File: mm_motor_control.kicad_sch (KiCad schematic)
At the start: 0 parts

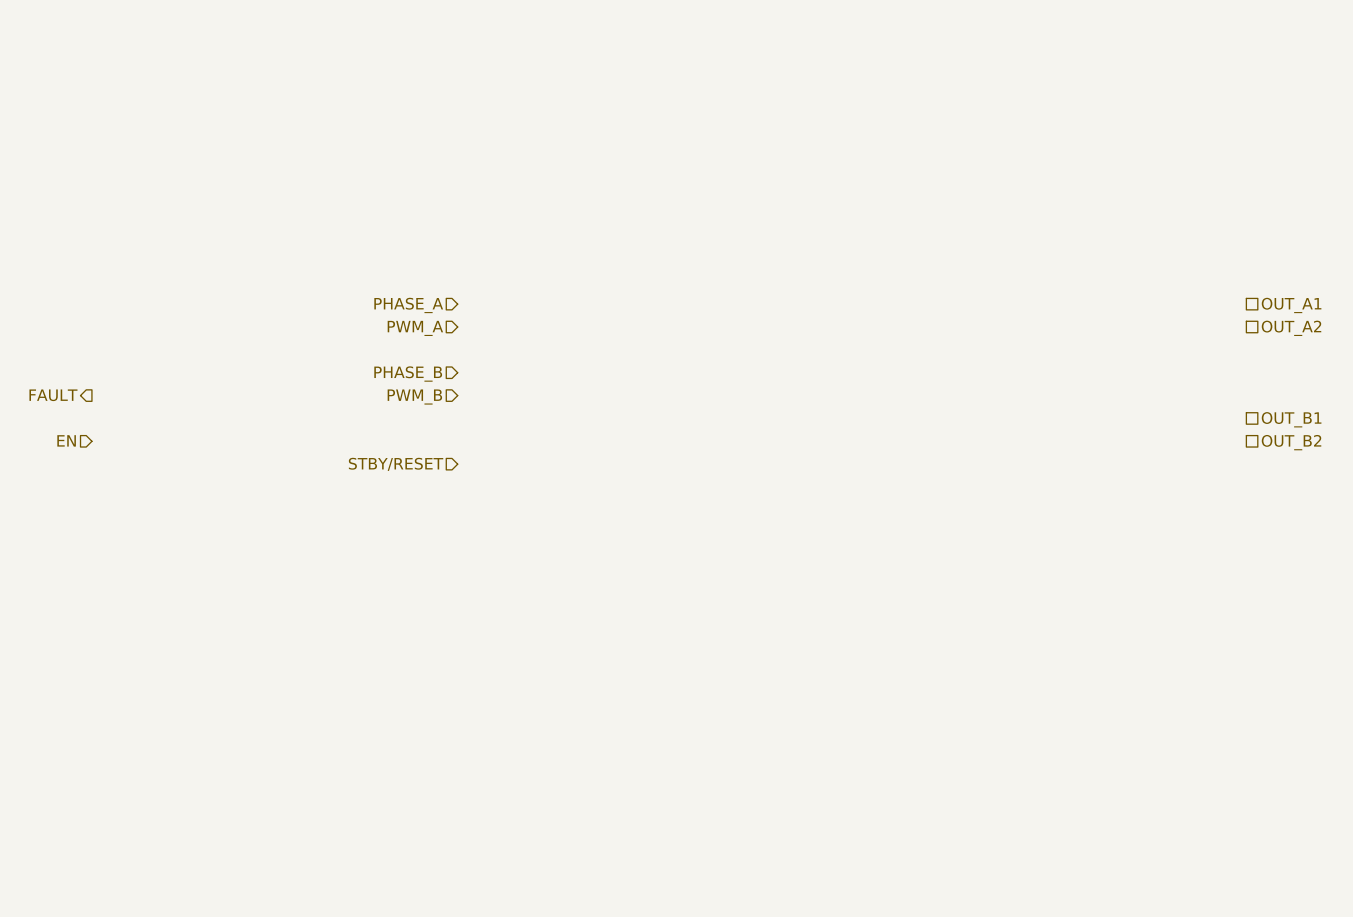
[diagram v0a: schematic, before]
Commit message: fin TP2
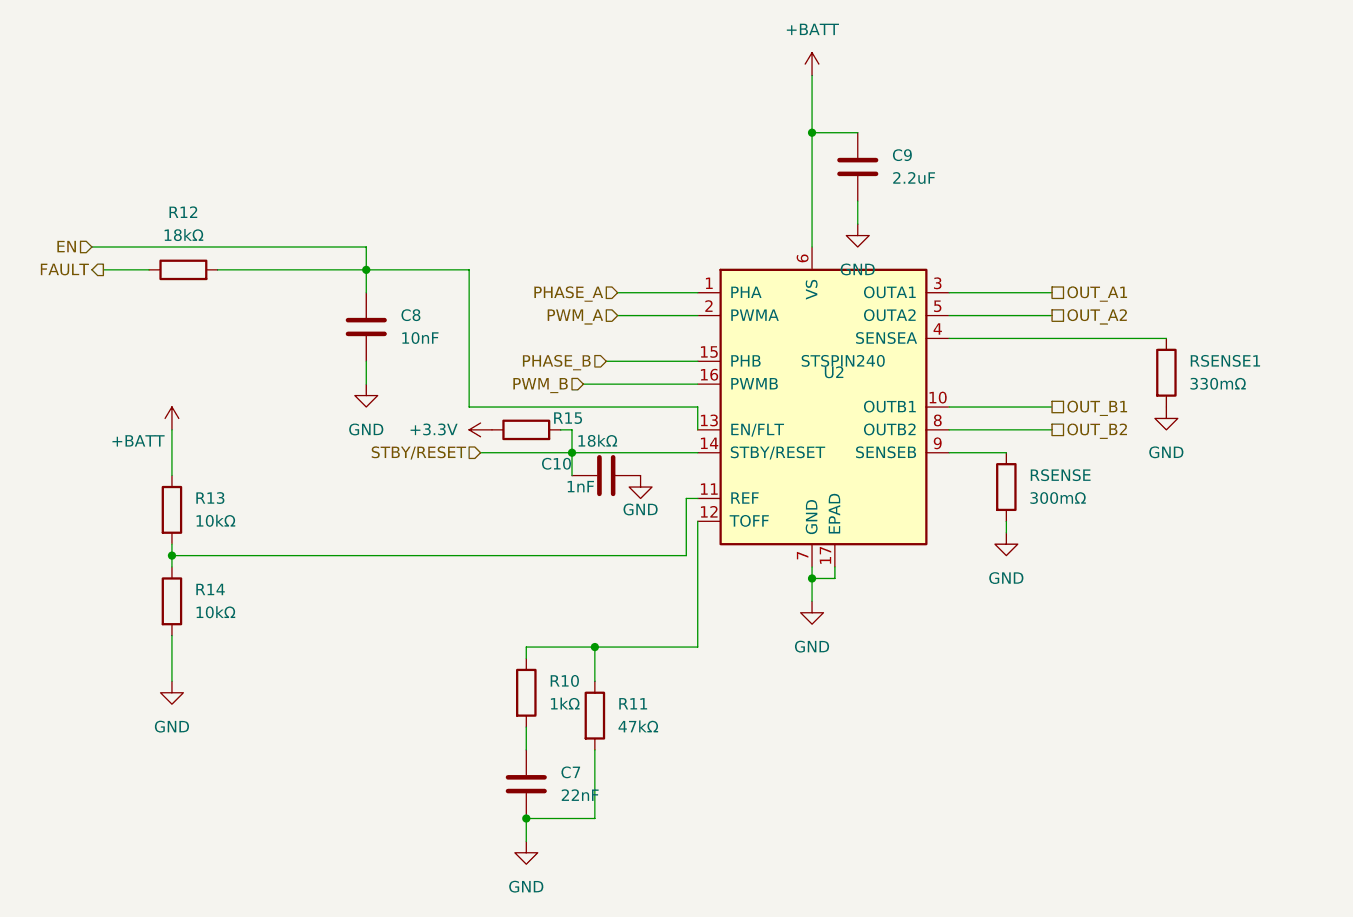
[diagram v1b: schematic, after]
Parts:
- added C10: 1nF, Capacitor_SMD:C_0603_1608Metric, symbol Device:C
- added C7: 22nF, Capacitor_SMD:C_0603_1608Metric, symbol Device:C
- added C8: 10nF, Capacitor_SMD:C_0603_1608Metric, symbol Device:C
- added C9: 2.2uF, Capacitor_SMD:C_0603_1608Metric, symbol Device:C
- added R10: 1kΩ, Resistor_SMD:R_0603_1608Metric, symbol Device:R
- added R11: 47kΩ, Resistor_SMD:R_0603_1608Metric, symbol Device:R
- added R12, R15: 18kΩ, Resistor_SMD:R_0603_1608Metric, symbol Device:R
- added R13, R14: 10kΩ, symbol Device:R
- added RSENSE: 300mΩ, Resistor_SMD:R_2512_6332Metric, symbol Device:R
- added RSENSE1: 330mΩ, Resistor_SMD:R_2512_6332Metric, symbol Device:R
- added U2: STSPIN240, Package_DFN_QFN:VQFN-16-1EP_3x3mm_P0.5mm_EP1.8x1.8mm, symbol Driver_Motor:STSPIN240
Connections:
- net EN: now also C8.1, R12.2, U2.13 (EN/FLT)
- net FAULT: now also R12.1
- net OUT_A1: now also U2.3 (OUTA1)
- net OUT_A2: now also U2.5 (OUTA2)
- net OUT_B1: now also U2.10 (OUTB1)
- net OUT_B2: now also U2.8 (OUTB2)
- net PHASE_A: now also U2.1 (PHA)
- net PHASE_B: now also U2.15 (PHB)
- net PWM_A: now also U2.2 (PWMA)
- net PWM_B: now also U2.16 (PWMB)
- net STBY/RESET: now also C10.1, R15.2, U2.14 (STBY/RESET)
- new net: R10.1, R11.1, U2.12 (TOFF)
- new net: C7.1, R10.2
- new net: RSENSE1.1, U2.4 (SENSEA)
- new net: R13.2, R14.1, U2.11 (REF)
- new net: RSENSE.1, U2.9 (SENSEB)
- new net +3.3V: R15.1
- new net +BATT: C9.1, R13.1, U2.6 (VS)
- new net GND: C10.2, C7.2, C8.2, C9.2, R11.2, R14.2, RSENSE.2, RSENSE1.2, U2.17 (EPAD), U2.7 (GND)
